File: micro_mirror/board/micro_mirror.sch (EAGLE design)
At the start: 37 parts, among them IC1 7407D, IC2 7402D, IC3 74S08D, IC4 LM324D

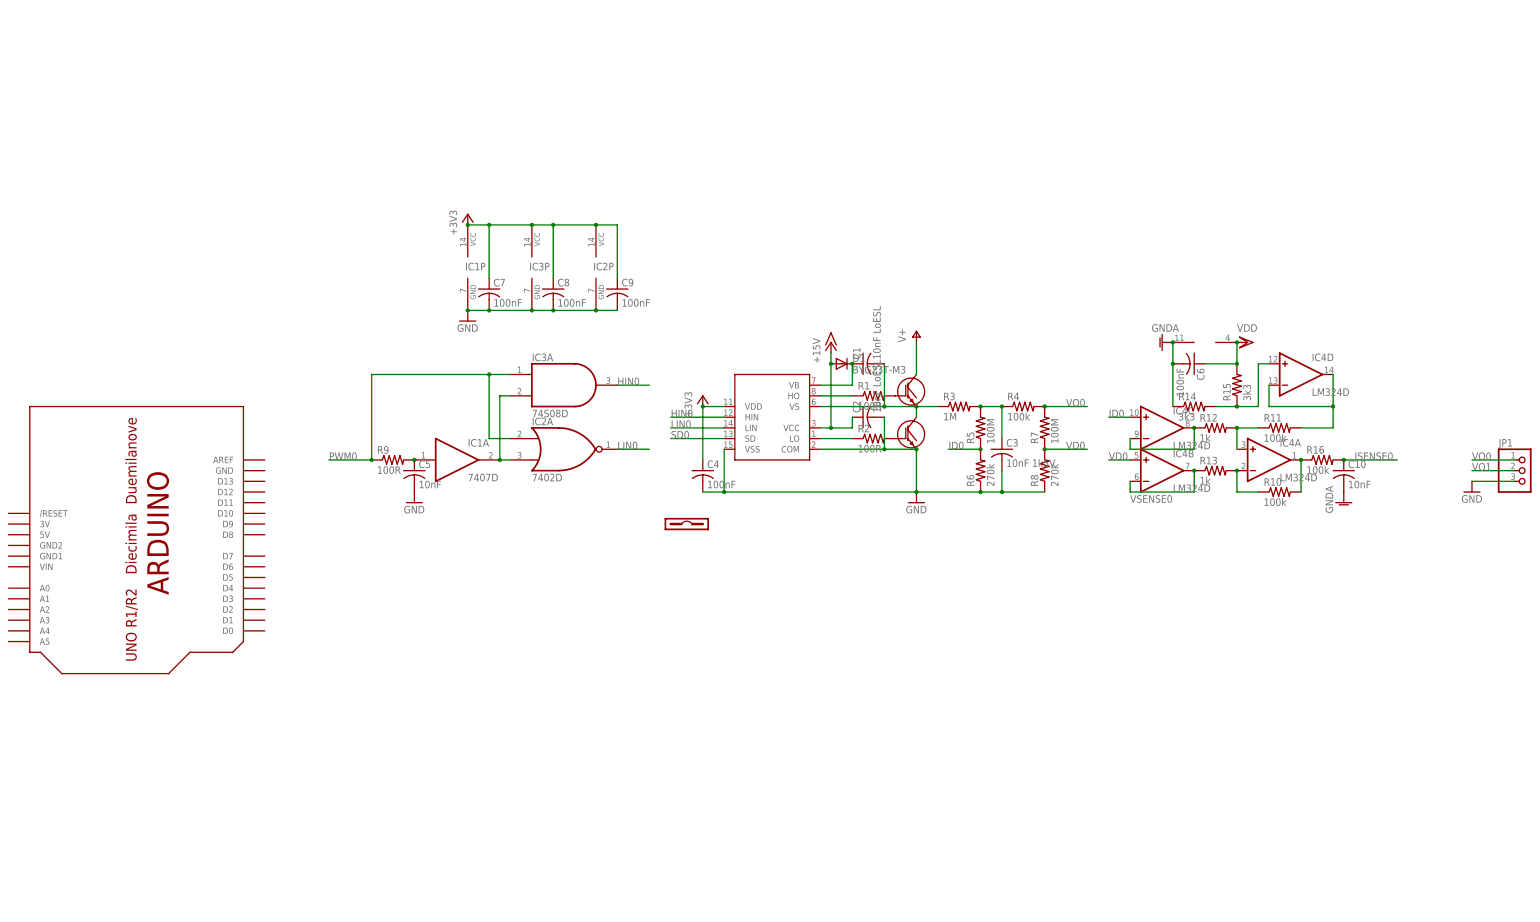
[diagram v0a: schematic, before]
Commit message: Layout pretty much done, need to do silkscreen.
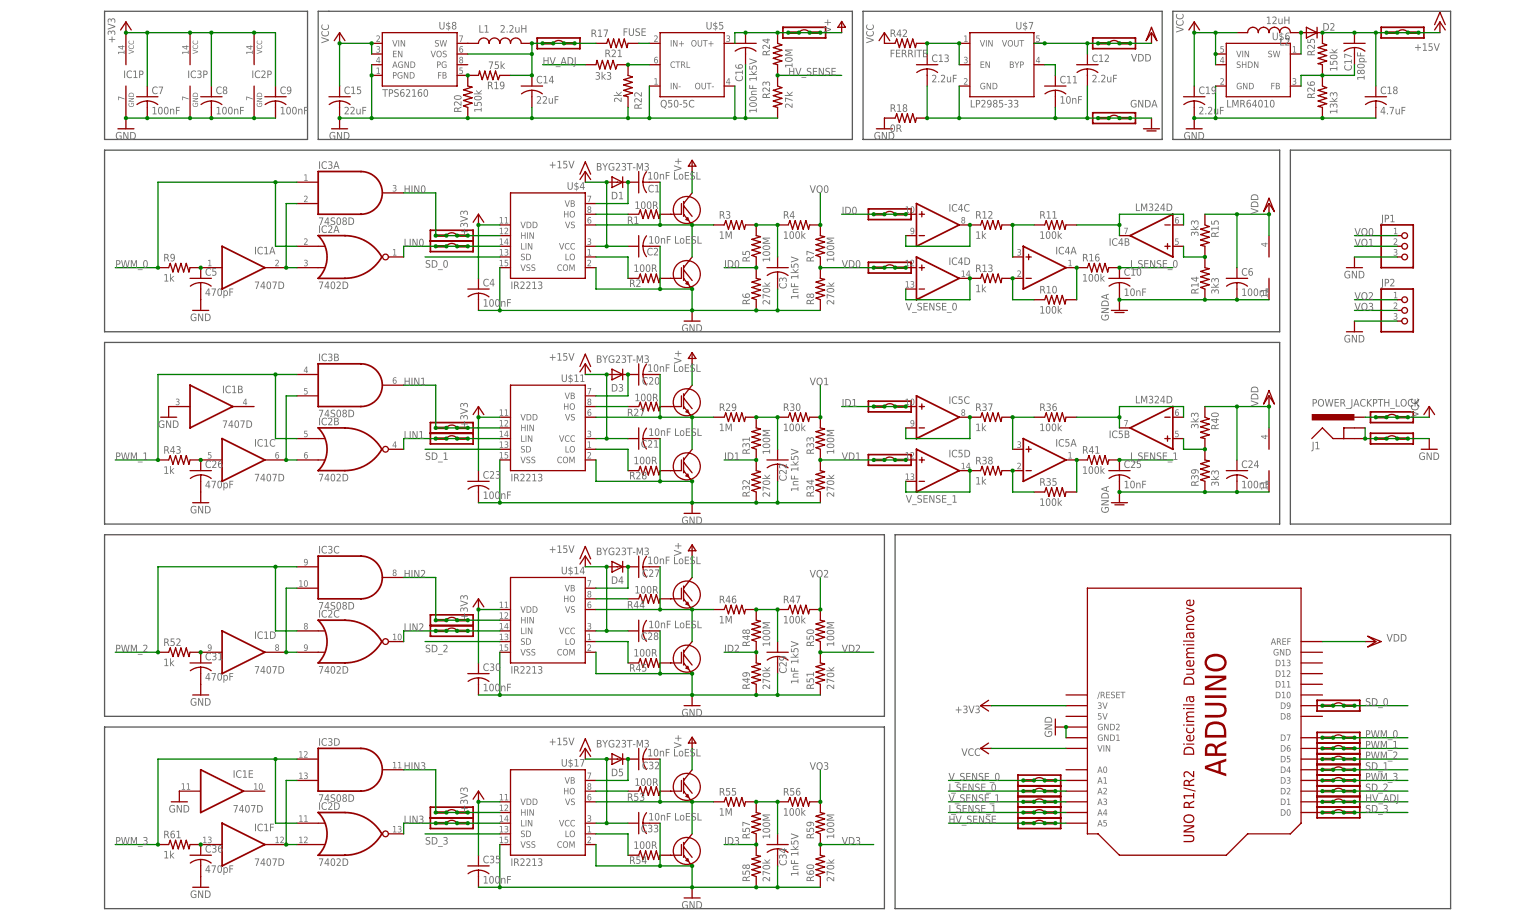
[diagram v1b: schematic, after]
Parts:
- added 15V_OUT, GND, GNDA, HIN0, HIN1, HIN2, HIN3, HV_ADJ, HV_IN, HV_OUT, HV_SENSE, ID0, ID1, I_SENSE_0, I_SENSE_1, LIN0, LIN1, LIN2, LIN3, PWM_0, PWM_1, PWM_2, PWM_3, SD_0, SD_1, SD_2, SD_3, VCC, VD0, VD1, VDDA, V_SENSE_0, V_SENSE_1: (no value), modular_robotics:M04LOCK
- added C11, C25: 10nF, rcl:C-USC1206
- added C12, C13, C19: 2.2uF, rcl:C-USC1206
- added C14, C15: 22uF, rcl:C-USC1206
- added C16: 100nF 1k5V, rcl:C-USC2225K
- added C17: 180pF, rcl:C-USC1206
- added C18: 4.7uF, rcl:C-USC1206
- added C20, C21, C27, C28, C32, C33: 10nF LoESL, rcl:C-USC1206
- added C22, C29, C34: 1nF 1k5V, rcl:C-USC1206
- added C23, C24, C30, C35: 100nF, rcl:C-USC1206
- added C26, C31, C36: 470pF, rcl:C-USC1206
- added D2: (no value), diode:DIODE-SOD123
- added D3, D4, D5: BYG23T-M3, diode:DIODE-DO214AC
- added IC5: LM324D, linear:LM324D
- added J1: POWER_JACKPTH_LOCK, SparkFun-Connectors:POWER_JACKPTH_LOCK
- added L1: 2.2uH, modular_robotics:INDUCTOR
- added L2: 12uH, rcl:L-USL1812
- added R17: FUSE, rcl:R-US_R1206
- added R18: 0R, rcl:R-US_R1206
- added R19: 75k, rcl:R-US_R1206
- added R20, R25: 150k, rcl:R-US_R1206
- added R21, R39, R40: 3k3, rcl:R-US_R1206
- added R22: 2k, rcl:R-US_R1206
- added R23: 27k, rcl:R-US_R1206
- added R24: 10M, rcl:R-US_R1206
- added R26: 13k3, rcl:R-US_R1206
- added R27, R28, R44, R45, R53, R54: 100R, rcl:R-US_R1206
- added R29, R46, R55: 1M, rcl:R-US_R1206
- added R30, R35, R36, R41, R47, R56: 100k, rcl:R-US_R1206
- added R31, R33, R48, R50, R57, R59: 100M, rcl:R-US_R1206
- added R32, R34, R49, R51, R58, R60: 270k, rcl:R-US_R1206
- added R37, R38, R43, R52, R61: 1k, rcl:R-US_R1206
- added R42: FERRITE, rcl:R-US_R1206
- added U$10, U$12, U$13, U$15, U$16, U$9: HGTD1N120BNS, modular_robotics:HGTD1N120BNS
- added U$11, U$14, U$17: IR2213, modular_robotics:IR2213
- added U$5: Q50-5C, modular_robotics:Q50-5C
- added U$6: LMR64010, modular_robotics:LMR64010
- added U$7: LP2985-33, modular_robotics:LP2985-33
- added U$8: TPS62160, modular_robotics:TPS62160
- C3: value 10nF 1k5V -> 1nF 1k5V
- C5: value 10nF -> 470pF
- JP2: device modular_robotics:M04LOCK -> pinhead:PINHD-1X3
- R9: value 100R -> 1k
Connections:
- removed net ISENSE0: C10.1, R16.2
- removed net PWM0: IC2A.I0, IC3A.I0, R9.1
- removed net SD0: U$4.SD
- removed net VSENSE0: IC4B.-IN, IC4B.OUT, R13.1
- new net HIN1: HIN1.1, HIN1.2, HIN1.3, HIN1.4, IC3B.O, U$11.HIN
- new net HIN2: HIN2.1, HIN2.2, HIN2.3, HIN2.4, IC3C.O, U$14.HIN
- new net HIN3: HIN3.1, HIN3.2, HIN3.3, HIN3.4, IC3D.O, U$17.HIN
- new net HV_ADJ: HV_ADJ.1, HV_ADJ.2, HV_ADJ.3, HV_ADJ.4, R21.2, U$1.D1
- new net HV_SENSE: HV_SENSE.1, HV_SENSE.2, HV_SENSE.3, HV_SENSE.4, R23.1, R24.2, U$1.A5
- new net ID1: IC5C.+IN, ID1.1, ID1.2, ID1.3, ID1.4, R31.1, R32.2
- new net ID2: R48.1, R49.2
- new net ID3: R57.1, R58.2
- new net I_SENSE_0: C10.1, I_SENSE_0.1, I_SENSE_0.2, I_SENSE_0.3, I_SENSE_0.4, R16.2, U$1.A2
- new net I_SENSE_1: C25.1, I_SENSE_1.1, I_SENSE_1.2, I_SENSE_1.3, I_SENSE_1.4, R41.2, U$1.A4
- new net LIN1: IC2B.O, LIN1.1, LIN1.2, LIN1.3, LIN1.4, U$11.LIN
- new net LIN2: IC2C.O, LIN2.1, LIN2.2, LIN2.3, LIN2.4, U$14.LIN
- new net LIN3: IC2D.O, LIN3.1, LIN3.2, LIN3.3, LIN3.4, U$17.LIN
- new net N$12: R17.2, U$5.IN+
- new net N$17: L1.1, U$8.SW
- new net N$18: C14.1, HV_IN.1, HV_IN.2, HV_IN.3, HV_IN.4, L1.2, R17.1, R19.1, U$8.VOS
- new net N$19: C11.1, U$7.BYP
- new net N$20: R19.2, R20.2, U$8.FB
- new net N$21: D2.A, L2.2, U$6.SW
- new net N$22: R27.2, U$9.G
- new net N$23: C17.2, R25.2, R26.1, U$6.FB
- new net N$24: R21.1, R22.1, U$5.CTRL
- new net N$25: R28.2, U$10.G
- new net N$26: C20.2, R29.1, U$10.C, U$11.VS, U$9.E
- new net N$27: R27.1, U$11.HO
- new net N$28: R28.1, U$11.LO
- new net N$29: C20.1, D3.C, U$11.VB
- new net N$30: C22.1, R29.2, R30.1, R31.2
- new net N$31: IC5C.-IN, IC5C.OUT, R37.1
- new net N$32: IC5A.-IN, R35.1, R38.2
- new net N$33: IC5A.+IN, R36.1, R37.2
- new net N$34: IC5B.-IN, IC5B.OUT, R36.2
- new net N$35: IC5A.OUT, R35.2, R41.1
- new net N$36: IC5B.+IN, R39.2, R40.2
- new net N$37: C13.1, R42.2, U$7.EN, U$7.VIN
- new net N$38: IC1C.O, IC2B.I1, IC3B.I1
- new net N$39: C26.1, IC1C.I, R43.2
- new net N$40: R44.2, U$12.G
- new net N$41: R45.2, U$13.G
- new net N$42: C27.2, R46.1, U$12.E, U$13.C, U$14.VS
- new net N$43: R44.1, U$14.HO
- new net N$44: R45.1, U$14.LO
- new net N$45: C27.1, D4.C, U$14.VB
- new net N$46: C29.1, R46.2, R47.1, R48.2
- new net N$47: IC1D.O, IC2C.I1, IC3C.I1
- new net N$48: R53.2, U$15.G
- new net N$49: C31.1, IC1D.I, R52.2
- new net N$50: R54.2, U$16.G
- new net N$51: C32.2, R55.1, U$15.E, U$16.C, U$17.VS
- new net N$52: R53.1, U$17.HO
- new net N$53: R54.1, U$17.LO
- new net N$54: C32.1, D5.C, U$17.VB
- new net N$55: C34.1, R55.2, R56.1, R57.2
- new net N$56: IC1F.O, IC2D.I1, IC3D.I1
- new net N$57: C36.1, IC1F.I, R61.2
- new net PWM_0: IC2A.I0, IC3A.I0, PWM_0.1, PWM_0.2, PWM_0.3, PWM_0.4, R9.1, U$1.D7
- new net PWM_1: IC2B.I0, IC3B.I0, PWM_1.1, PWM_1.2, PWM_1.3, PWM_1.4, R43.1, U$1.D6
- new net PWM_2: IC2C.I0, IC3C.I0, PWM_2.1, PWM_2.2, PWM_2.3, PWM_2.4, R52.1, U$1.D5
- new net PWM_3: IC2D.I0, IC3D.I0, PWM_3.1, PWM_3.2, PWM_3.3, PWM_3.4, R61.1, U$1.D3
- new net SD_0: SD_0.1, SD_0.2, SD_0.3, SD_0.4, U$1.D9, U$4.SD
- new net SD_1: SD_1.1, SD_1.2, SD_1.3, SD_1.4, U$1.D4, U$11.SD
- new net SD_2: SD_2.1, SD_2.2, SD_2.3, SD_2.4, U$1.D2, U$14.SD
- new net SD_3: SD_3.1, SD_3.2, SD_3.3, SD_3.4, U$1.D0, U$17.SD
- new net VCC: C15.1, C19.1, J1.PWR, L2.1, R42.1, U$1.VIN, U$6.SHDN, U$6.VIN, U$8.EN, U$8.VIN, VCC.1, VCC.2, VCC.3, VCC.4
- new net VD1: IC5D.+IN, R33.1, R34.2, VD1.1, VD1.2, VD1.3, VD1.4
- new net VD2: R50.1, R51.2
- new net VD3: R59.1, R60.2
- new net VO2: JP2.1, R47.2, R50.2
- new net VO3: JP2.2, R56.2, R59.2
- new net V_SENSE_0: IC4D.-IN, IC4D.OUT, R13.1, U$1.A1, V_SENSE_0.1, V_SENSE_0.2, V_SENSE_0.3, V_SENSE_0.4
- new net V_SENSE_1: IC5D.-IN, IC5D.OUT, R38.1, U$1.A3, V_SENSE_1.1, V_SENSE_1.2, V_SENSE_1.3, V_SENSE_1.4
- net +15V: now also 15V_OUT.1, 15V_OUT.2, 15V_OUT.3, 15V_OUT.4, C17.1, C18.1, C21.1, C28.1, C33.1, D2.C, D3.A, D4.A, D5.A, R25.1, U$11.VCC, U$14.VCC, U$17.VCC
- net +3V3: now also C23.1, C30.1, C35.1, U$1.3V, U$11.VDD, U$14.VDD, U$17.VDD
- net GND: now also C14.2, C15.2, C16.2, C18.2, C19.2, C21.2, C22.2, C23.2, C26.2, C28.2, C29.2, C30.2, C31.2, C33.2, C34.2, C35.2, C36.2, GND.1, GND.2, GND.3, GND.4, IC1B.I, IC1E.I, J1.GND, J1.GNDBREAK, JP2.3, R18.1, R20.1, R22.2, R23.2, R26.2, R32.1, R34.1, R49.1, R51.1, R58.1, R60.1, U$1.GND1, U$1.GND2, U$10.E, U$11.COM, U$11.VSS, U$13.E, U$14.COM, U$14.VSS, U$16.E, U$17.COM, U$17.VSS, U$5.IN-, U$5.OUT-, U$6.GND, U$8.AGND, U$8.PGND
- net GNDA: now also C11.2, C12.2, C13.2, C24.2, C25.2, GNDA.1, GNDA.2, GNDA.3, GNDA.4, IC5P.V-, R18.2, R39.1, U$7.GND
- net HIN0: now also HIN0.1, HIN0.2, HIN0.3, HIN0.4
- net ID0: now also ID0.1, ID0.2, ID0.3, ID0.4
- net LIN0: now also LIN0.1, LIN0.2, LIN0.3, LIN0.4
- net N$15: now also IC4B.+IN, R15.2; no longer IC4D.+IN, R15.1
- net N$16: now also IC4B.-IN, IC4B.OUT; no longer IC4D.-IN, IC4D.OUT
- net V+: now also C16.1, HV_OUT.1, HV_OUT.2, HV_OUT.3, HV_OUT.4, R24.1, U$12.C, U$15.C, U$5.OUT+, U$9.C
- net VD0: now also IC4D.+IN, VD0.1, VD0.2, VD0.3, VD0.4; no longer IC4B.+IN
- net VDD: now also C12.1, C24.1, IC5P.V+, R15.1, R40.1, U$1.AREF, U$7.VOUT, VDDA.1, VDDA.2, VDDA.3, VDDA.4; no longer R15.2
- net VO1: now also R30.2, R33.2
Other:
- moved on the sheet: C1, C10, C2, C3, C4, C5, C6, C7, C8, C9, D1, IC1A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
